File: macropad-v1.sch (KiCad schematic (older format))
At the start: 24 parts, among them SW1 SW_Push, U1 ATmega32U4-AU, Y1 16MHz

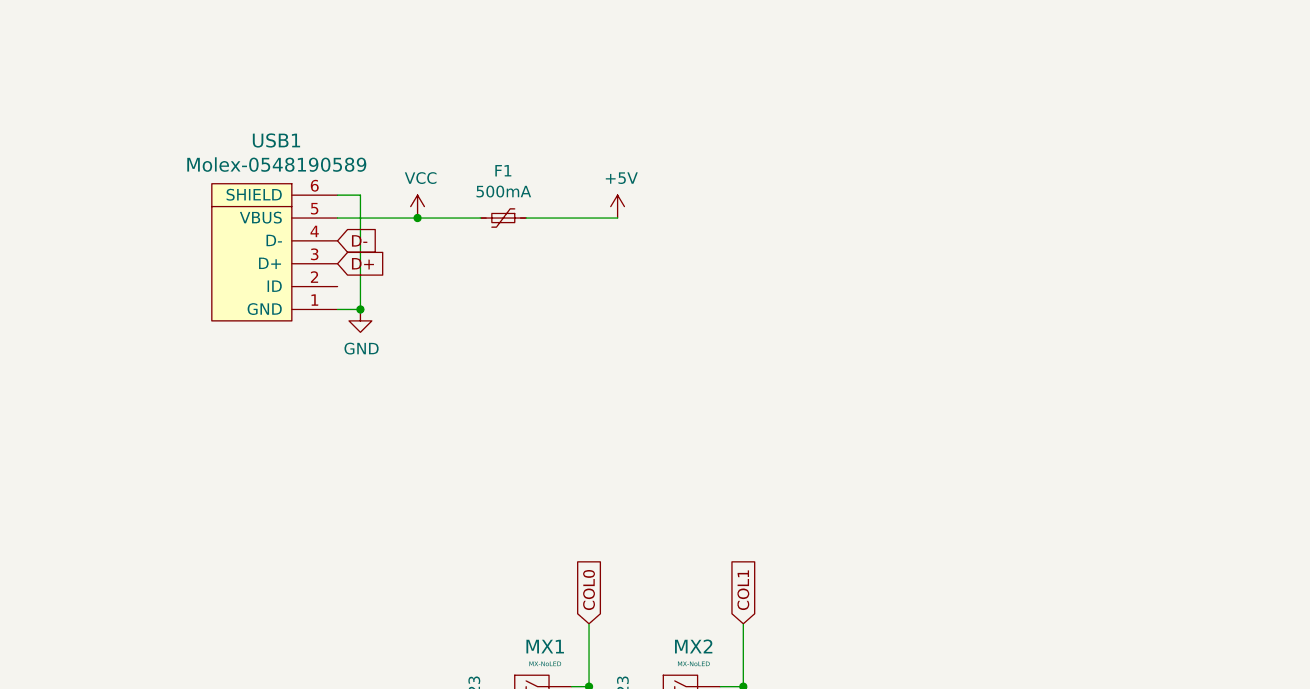
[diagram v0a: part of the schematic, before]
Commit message: usb c v1
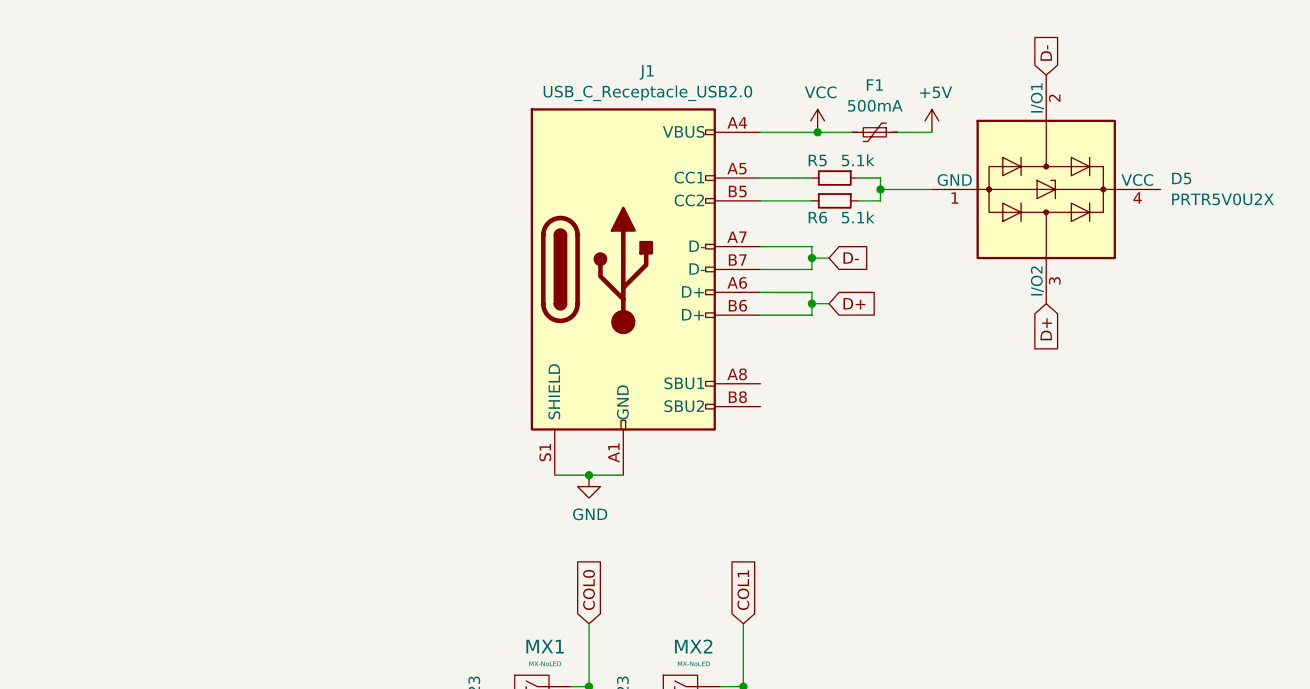
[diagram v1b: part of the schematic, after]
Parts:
- removed USB1: Molex-0548190589, random-keyboard-parts:Molex-0548190589, symbol random-keyboard-parts:Molex-0548190589
- added D5: PRTR5V0U2X, Package_TO_SOT_SMD:SOT-143, symbol Power_Protection:PRTR5V0U2X
- added J1: USB_C_Receptacle_USB2.0, Connector_USB:USB_C_Receptacle_Amphenol_12401548E4-2A, symbol Connector:USB_C_Receptacle_USB2.0
- added R5, R6: 5.1k, Resistor_SMD:R_0805_2012Metric, symbol Device:R_Small
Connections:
- net D+: now also D5.3 (I/O2), J1.A6 (D+), J1.B6 (D+)
- net D-: now also D5.2 (I/O1), J1.A7 (D-), J1.B7 (D-)
- net GND: now also J1.A1 (GND), J1.A12 (GND), J1.B1 (GND), J1.B12 (GND), J1.S1 (SHIELD)
- net VCC: now also J1.A4 (VBUS), J1.A9 (VBUS), J1.B4 (VBUS), J1.B9 (VBUS)
- new net: J1.A5 (CC1), R5.2
- new net: J1.B5 (CC2), R6.2
- new net: D5.1 (GND), R5.1, R6.1
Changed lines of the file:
@@
 D-
-$Comp
-L random-keyboard-parts:Molex-0548190589 USB1
-U 1 1 5F4FAE8C
-P 6525 1475
-F 0 "USB1" V 7062 1442 60  0000 C CNN
-F 1 "Molex-0548190589" V 6956 1442 60  0000 C CNN
-F 2 "random-keyboard-parts:Molex-0548190589" H 6525 1475 60  0001 C CNN
-F 3 "" H 6525 1475 60  0001 C CNN
-	1    6525 1475
-	0    -1   -1   0
-$EndComp
-$Comp
-L Device:Polyfuse_Small F1
-U 1 1 5F4FEAD4
-P 7550 1275
-F 0 "F1" V 7345 1275 50  0000 C CNN
-F 1 "500mA" V 7436 1275 50  0000 C CNN
-F 2 "Fuse:Fuse_1206_3216Metric" H 7600 1075 50  0001 L CNN
-F 3 "~" H 7550 1275 50  0001 C CNN
-	1    7550 1275
-	0    1    1    0
-$EndComp
-$Comp
-L power:+5V #PWR0111
-U 1 1 5F500AF0
-P 8050 1275
-F 0 "#PWR0111" H 8050 1125 50  0001 C CNN
-F 1 "+5V" H 8065 1448 50  0000 C CNN
-F 2 "" H 8050 1275 50  0001 C CNN
-F 3 "" H 8050 1275 50  0001 C CNN
-	1    8050 1275
-	1    0    0    -1
-$EndComp
-$Comp
-L power:VCC #PWR0112
-U 1 1 5F506E8B
-P 7175 1275
-F 0 "#PWR0112" H 7175 1125 50  0001 C CNN
-F 1 "VCC" H 7190 1448 50  0000 C CNN
-F 2 "" H 7175 1275 50  0001 C CNN
-F 3 "" H 7175 1275 50  0001 C CNN
-	1    7175 1275
-	1    0    0    -1
-$EndComp
-Wire Wire Line
-	8050 1275 7650 1275
-Wire Wire Line
-	7450 1275 7175 1275
-Wire Wire Line
-	7175 1275 6825 1275
-Connection ~ 7175 1275
-Text GLabel 6825 1375 2    50   Input ~ 0
-D-
-Text GLabel 6825 1475 2    50   Input ~ 0
-D+
-$Comp
-L power:GND #PWR0113
-U 1 1 5F50A9D7
-P 6925 1675
-F 0 "#PWR0113" H 6925 1425 50  0001 C CNN
-F 1 "GND" H 6930 1502 50  0000 C CNN
-F 2 "" H 6925 1675 50  0001 C CNN
-F 3 "" H 6925 1675 50  0001 C CNN
-	1    6925 1675
-	1    0    0    -1
-$EndComp
-Wire Wire Line
-	6925 1675 6825 1675
 $Comp
 L Device:D_Small D1
@@
 Text GLabel 4900 3725 2    50   Input ~ 0
 ROW1
-Wire Wire Line
-	6825 1175 6925 1175
-Wire Wire Line
-	6925 1175 6925 1675
-Connection ~ 6925 1675
+$Comp
+L Connector:USB_C_Receptacle_USB2.0 J1
+U 1 1 5F500470
+P 8075 1500
+F 0 "J1" H 8182 2367 50  0000 C CNN
+F 1 "USB_C_Receptacle_USB2.0" H 8182 2276 50  0000 C CNN
+F 2 "Connector_USB:USB_C_Receptacle_Amphenol_12401548E4-2A" H 8225 1500 50  0001 C CNN
+F 3 "https://www.usb.org/sites/default/files/documents/usb_type-c.zip" H 8225 1500 50  0001 C CNN
+	1    8075 1500
+	1    0    0    -1
+$EndComp
+$Comp
+L power:GND #PWR03
+U 1 1 5F502EF6
+P 7925 2400
+F 0 "#PWR03" H 7925 2150 50  0001 C CNN
+F 1 "GND" H 7930 2227 50  0000 C CNN
+F 2 "" H 7925 2400 50  0001 C CNN
+F 3 "" H 7925 2400 50  0001 C CNN
+	1    7925 2400
+	1    0    0    -1
+$EndComp
+Wire Wire Line
+	7775 2400 7925 2400
+Connection ~ 7925 2400
+Wire Wire Line
+	7925 2400 8075 2400
+$Comp
+L power:VCC #PWR01
+U 1 1 5F50505C
+P 8925 900
+F 0 "#PWR01" H 8925 750 50  0001 C CNN
+F 1 "VCC" H 8940 1073 50  0000 C CNN
+F 2 "" H 8925 900 50  0001 C CNN
+F 3 "" H 8925 900 50  0001 C CNN
+	1    8925 900
+	1    0    0    -1
+$EndComp
+$Comp
+L Device:Polyfuse_Small F1
+U 1 1 5F505EC8
+P 9175 900
+F 0 "F1" V 8970 900 50  0000 C CNN
+F 1 "500mA" V 9061 900 50  0000 C CNN
+F 2 "Fuse:Fuse_1206_3216Metric" H 9225 700 50  0001 L CNN
+F 3 "~" H 9175 900 50  0001 C CNN
+	1    9175 900
+	0    1    1    0
+$EndComp
+Wire Wire Line
+	8675 900  8925 900
+Connection ~ 8925 900
+Wire Wire Line
+	8925 900  9075 900
+$Comp
+L power:+5V #PWR02
+U 1 1 5F508A84
+P 9425 900
+F 0 "#PWR02" H 9425 750 50  0001 C CNN
+F 1 "+5V" H 9440 1073 50  0000 C CNN
+F 2 "" H 9425 900 50  0001 C CNN
+F 3 "" H 9425 900 50  0001 C CNN
+	1    9425 900
+	1    0    0    -1
+$EndComp
+Wire Wire Line
+	9275 900  9425 900
+Wire Wire Line
+	8675 1400 8900 1400
+Wire Wire Line
+	8675 1500 8900 1500
+Wire Wire Line
+	8900 1400 8900 1450
+Wire Wire Line
+	8675 1600 8900 1600
+Wire Wire Line
+	8675 1700 8900 1700
+Wire Wire Line
+	8900 1600 8900 1650
+Wire Wire Line
+	8900 1450 8975 1450
+Connection ~ 8900 1450
+Wire Wire Line
+	8900 1450 8900 1500
+Wire Wire Line
+	8900 1650 8975 1650
+Connection ~ 8900 1650
+Wire Wire Line
+	8900 1650 8900 1700
+Text GLabel 8975 1450 2    50   Input ~ 0
+D-
+Text GLabel 8975 1650 2    50   Input ~ 0
+D+
+$Comp
+L Power_Protection:PRTR5V0U2X D5
+U 1 1 5F526AAB
+P 9925 1150
+F 0 "D5" V 9879 1694 50  0000 L CNN
+F 1 "PRTR5V0U2X" V 9970 1694 50  0000 L CNN
+F 2 "Package_TO_SOT_SMD:SOT-143" H 9985 1150 50  0001 C CNN
+F 3 "https://assets.nexperia.com/documents/data-sheet/PRTR5V0U2X.pdf" H 9985 1150 50  0001 C CNN
+	1    9925 1150
+	0    1    1    0
+$EndComp
+$Comp
+L Device:R_Small R5
+U 1 1 5F52842B
+P 9000 1100
+F 0 "R5" V 8925 1025 50  0000 C CNN
+F 1 "5.1k" V 8925 1200 50  0000 C CNN
+F 2 "Resistor_SMD:R_0805_2012Metric" H 9000 1100 50  0001 C CNN
+F 3 "~" H 9000 1100 50  0001 C CNN
+	1    9000 1100
+	0    1    1    0
+$EndComp
+$Comp
+L Device:R_Small R6
+U 1 1 5F529414
+P 9000 1200
+F 0 "R6" V 9075 1125 50  0000 C CNN
+F 1 "5.1k" V 9075 1300 50  0000 C CNN
+F 2 "Resistor_SMD:R_0805_2012Metric" H 9000 1200 50  0001 C CNN
+F 3 "~" H 9000 1200 50  0001 C CNN
+	1    9000 1200
+	0    1    1    0
+$EndComp
+Wire Wire Line
+	8675 1100 8900 1100
+Wire Wire Line
+	8675 1200 8900 1200
+Wire Wire Line
+	9100 1100 9200 1100
+Wire Wire Line
+	9200 1100 9200 1150
+Wire Wire Line
+	9200 1200 9100 1200
+Wire Wire Line
+	9200 1150 9425 1150
+Connection ~ 9200 1150
+Wire Wire Line
+	9200 1150 9200 1200
+Text GLabel 9925 650  1    50   Input ~ 0
+D-
+Text GLabel 9925 1650 3    50   Input ~ 0
+D+
 $EndSCHEMATC
